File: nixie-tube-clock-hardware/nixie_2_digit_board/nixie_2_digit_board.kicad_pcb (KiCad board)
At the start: 2 copper layers, 100 x 47 mm, 99 parts, among them J1 Conn_01x05, J2 Dot Connection, J3 GPIO in for dot, P1 CONN_01X01, P3 CONN_01X01, Q1 MPSA42, U1 570Nixie, U10 570Nixie, U11 SN74141-BCD-DEC-DECODE, U2 SN74141-BCD-DEC-DECODE, U3 SN43HC595, U4 570Nixie, U5 SN74141-BCD-DEC-DECODE, U6 Logo, U7 570Nixie, U8 SN74141-BCD-DEC-DECODE, U9 SN43HC595

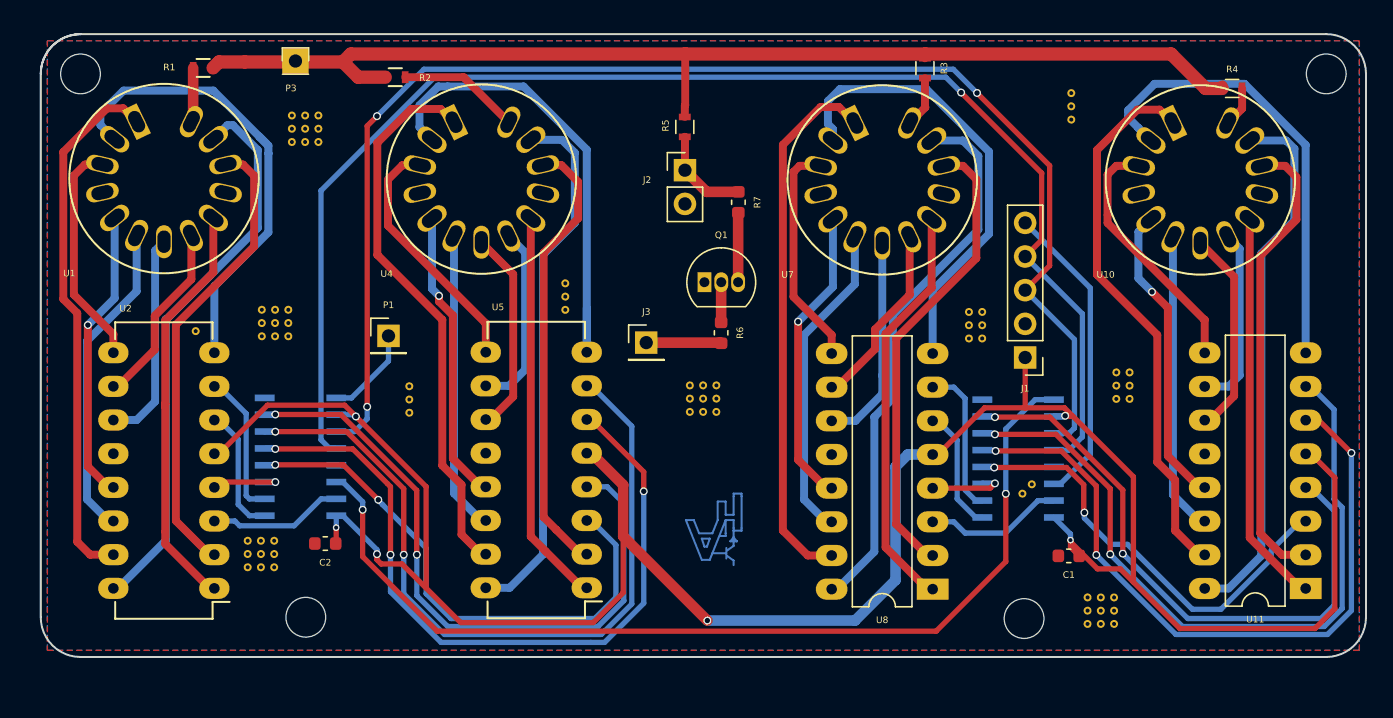
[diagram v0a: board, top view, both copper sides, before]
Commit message: V1.2 Control board
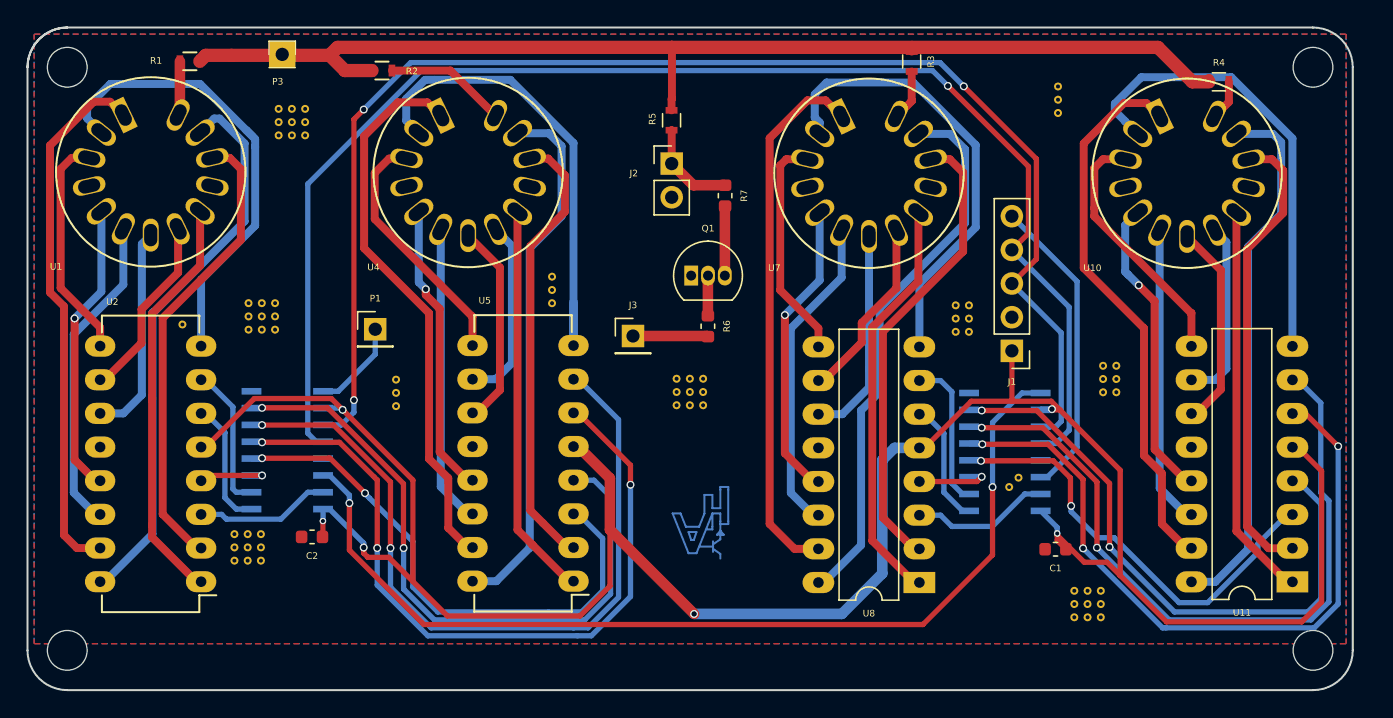
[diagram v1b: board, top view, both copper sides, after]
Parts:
- moved REF** 21.9 mm to (209.0, 110.5)
- moved REF** 18.2 mm to (115.0, 110.5)
- moved REF** 1.12 mm to (127.6, 101.7)
- moved REF** 1.12 mm to (127.6, 102.7)
- moved REF** 1.12 mm to (127.6, 103.7)
- moved C1 1.12 mm to (189.6, 102.9)
- moved C2 1.12 mm to (133.5, 101.9)
- moved J1 1.12 mm to (186.3, 87.9)
- moved J2 1.12 mm to (160.6, 73.8)
- moved J3 1.12 mm to (157.7, 86.8)
- moved P1 1.12 mm to (138.2, 86.3)
- moved P3 1.12 mm to (131.2, 65.5)
- moved Q1 1.12 mm to (162.1, 82.2)
- moved R1 1.12 mm to (124.2, 66.0)
- moved R2 1.12 mm to (138.8, 66.8)
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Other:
- board size 100 x 47 mm -> 100 x 50 mm
- net class Default removed
